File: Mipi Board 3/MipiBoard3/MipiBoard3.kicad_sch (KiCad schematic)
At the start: 51 parts, among them J1 Power/Control Top, J2 Bank A Top, J3 Bank B Top, J4 MIPI1, J5 MIPI2, J6 Bank A Bottom, J7 Bank B Bottom, J8 Power/Control Bottom, U1 LM339, U2 LM339, U3 LM339

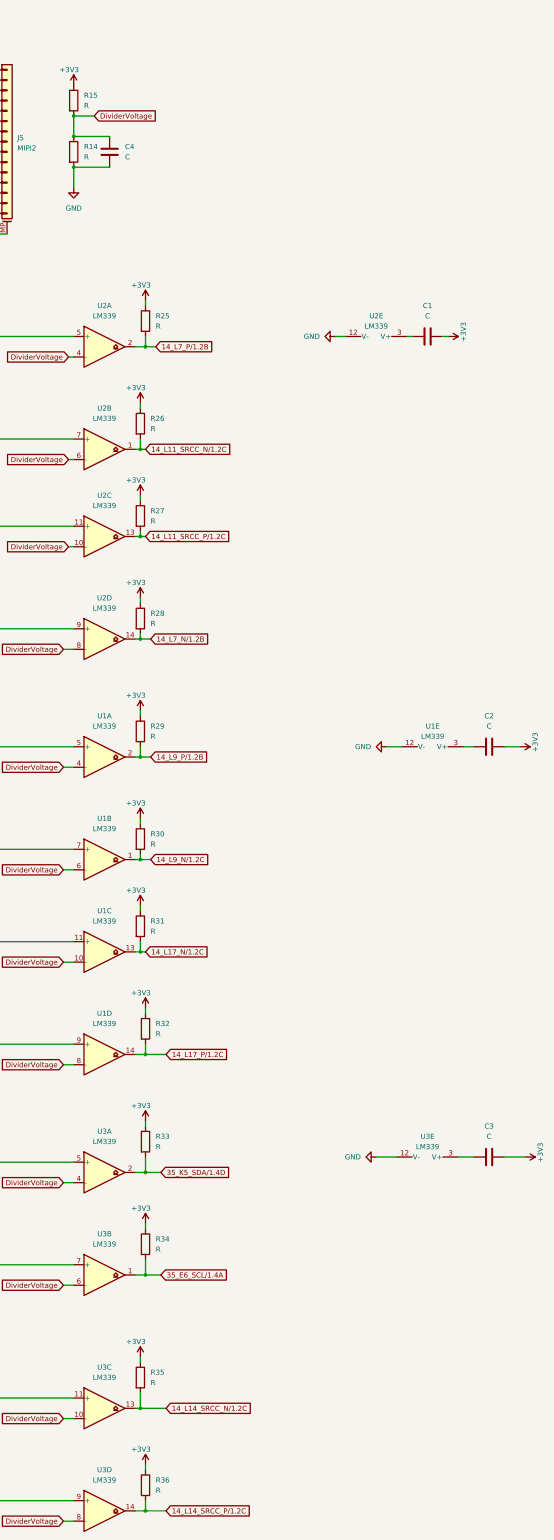
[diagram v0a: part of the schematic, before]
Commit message: Components layedout
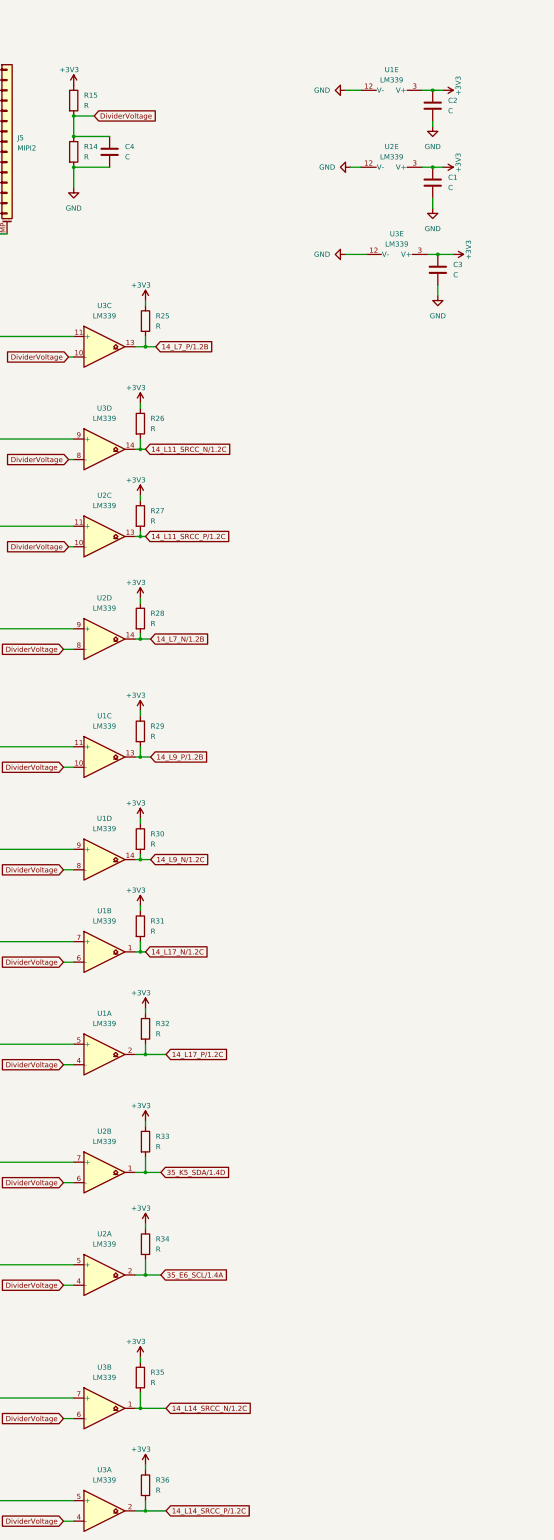
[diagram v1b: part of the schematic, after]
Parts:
- removed unit 2 of U3
- removed unit 1 of U3
- added unit 1 of U2
- added unit 2 of U2
- C1, C2, C3, C4: footprint (none) -> Capacitor_SMD:C_0201_0603Metric
- R14, R15: footprint Resistor_SMD:R_0805_2012Metric -> Resistor_SMD:R_0603_1608Metric
- R25, R26, R27, R28, R29, R30, R31, R32, R33, R34, R35, R36: footprint Resistor_SMD:R_0402_1005Metric -> Resistor_SMD:R_0603_1608Metric
- U1, U2, U3: footprint (none) -> Package_SO:TSSOP-14-1EP_4.4x5mm_P0.65mm
- U3: renamed from U2; footprint (none) -> Package_SO:TSSOP-14-1EP_4.4x5mm_P0.65mm
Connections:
- net +3V3: now also C1.2, C2.2, U1.3 (V+), U2.3 (V+), U3.3 (V+); no longer C1.1, C2.1
- net 14_L11_SRCC_N/1.2C: now also U3.14; no longer U3.1
- net 14_L14_SRCC_N/1.2C: now also U3.1; no longer U3.13
- net 14_L14_SRCC_P/1.2C: now also U3.2; no longer U3.14
- net 14_L17_N/1.2C: now also U1.1; no longer U1.13
- net 14_L17_P/1.2C: now also U1.2; no longer U1.14
- net 14_L7_P/1.2B: now also U3.13; no longer U3.2
- net 14_L9_N/1.2C: now also U1.14; no longer U1.1
- net 14_L9_P/1.2B: now also U1.13; no longer U1.2
- net 35_E6_SCL/1.4A: now also U2.2
- net 35_K5_SDA/1.4D: now also U2.1
- net DividerVoltage: now also U1.10 (-), U1.4 (-), U1.6 (-), U1.8 (-), U3.10 (-), U3.4 (-), U3.6 (-), U3.8 (-), U2.4 (-), U2.6 (-); no longer U1.10 (-), U1.4 (-), U1.6 (-), U1.8 (-), U3.10 (-), U3.4 (-), U3.6 (-), U3.8 (-)
- net GND: now also C1.1, C2.1, C3.2
- net at R23.1: now also U2.5 (+)
- net at R17.1: now also U2.7 (+)
- net at R12.1: now also U1.11 (+); no longer U1.5 (+)
- net at R18.1: now also U3.7 (+); no longer U3.11 (+)
- net at R16.1: now also U1.7 (+); no longer U1.11 (+)
- net at R22.1: now also U1.5 (+); no longer U1.9 (+)
- net at R21.1: now also U1.9 (+); no longer U1.7 (+)
- net at R19.1: now also U3.9 (+); no longer U3.7 (+)
- net at R24.1: now also U3.5 (+); no longer U3.9 (+)
- net at R6.1: now also U3.11 (+); no longer U3.5 (+)
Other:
- moved on the sheet: C1, C2, C3, U1E, U3E
